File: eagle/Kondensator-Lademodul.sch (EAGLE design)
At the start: 12 parts, among them X1 MKDSN1,5/2-5,08, X2 MKDSN1,5/2-5,08

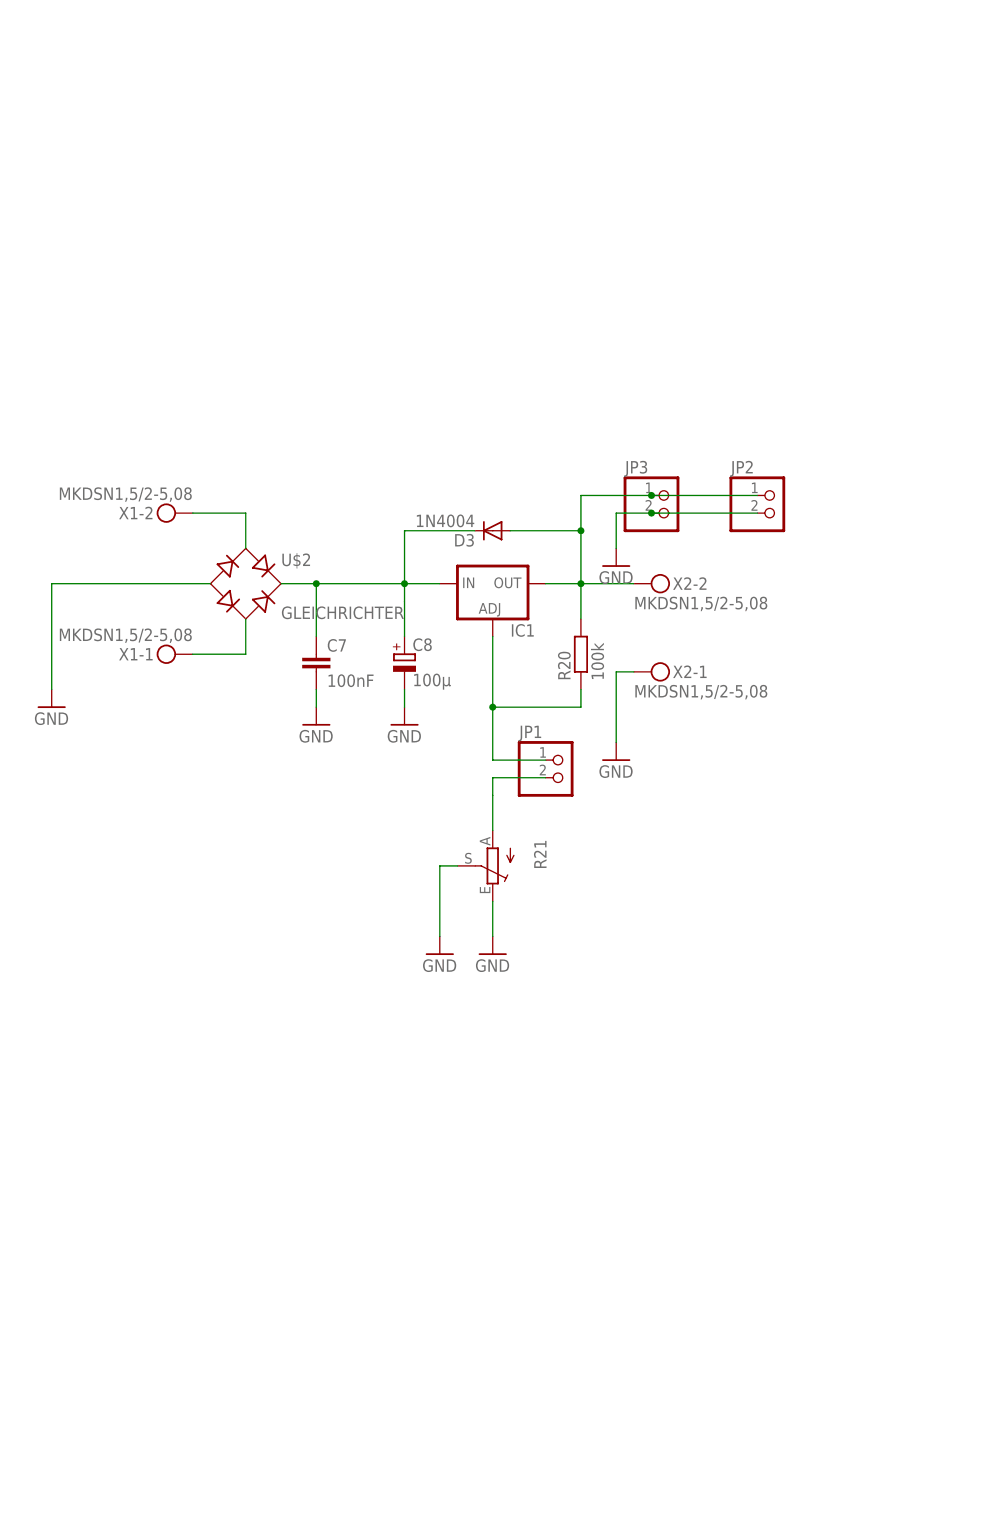
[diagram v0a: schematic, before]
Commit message: pcb design
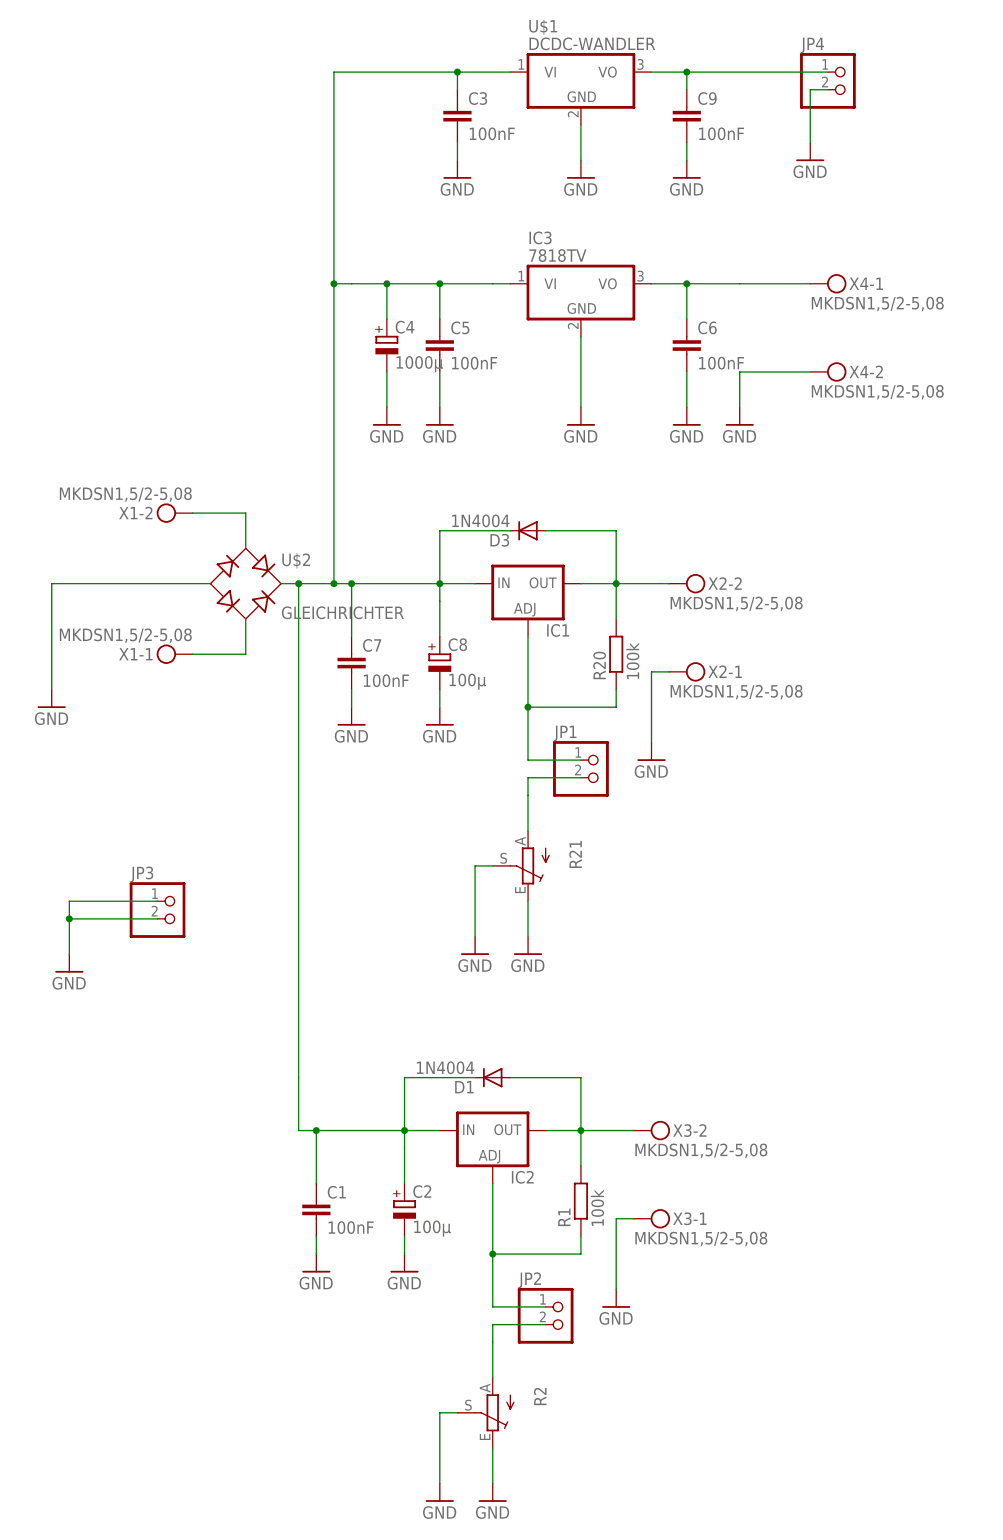
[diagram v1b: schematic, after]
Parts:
- added C1, C3, C5, C6, C9: 100nF, rcl:C-EUC0805
- added C2: 100µ, rcl:CPOL-EUE3.5-8
- added C4: 1000µ, rcl:CPOL-EUE3.5-8
- added D1: 1N4004, diode:1N4004
- added IC2: (no value), v-reg:LM317TS
- added IC3: 7818TV, linear:7805TV
- added JP4: (no value), pinhead:PINHD-1X2
- added R1: 100k, rcl:R-EU_R1206
- added R2: (no value), pot:TRIM_EU-PT10
- added U$1: DCDC-WANDLER, 0liver:DCDC-WANDLER
- added X3, X4: MKDSN1,5/2-5,08, con-phoenix-508:MKDSN1,5/2-5,08
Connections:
- removed net N$27: C7.1, C8.+, D3.C, IC1.IN, U$2.+
- new net N$17: C1.1, C2.+, C3.1, C4.+, C5.1, C7.1, C8.+, D1.C, D3.C, IC1.IN, IC2.IN, IC3.VI, U$1.VI, U$2.+
- new net N$2: C6.1, IC3.VO, X4-1.KL
- new net N$3: D1.A, IC2.OUT, R1.2, X3-2.KL
- new net N$4: IC2.ADJ, JP2.1, R1.1
- new net N$5: JP2.2, R2.A
- new net N$6: C9.1, JP4.1, U$1.VO
- net GND: now also C1.2, C2.-, C3.2, C4.-, C5.2, C6.2, C9.2, IC3.GND, JP3.1, JP4.2, R2.E, R2.S, U$1.GND, X3-1.KL, X4-2.KL; no longer JP2.2
- net N$28: no longer JP2.1, JP3.1
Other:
- moved on the sheet: C7, C8, D3, IC1, JP1, JP2, JP3, R20, R21, X2-1, X2-2
